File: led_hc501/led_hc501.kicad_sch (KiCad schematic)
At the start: 14 parts, among them J1 LED02, J10 Conn_01x03_Pin, J11 BATTERY, J2 Conn_01x01_Pin, J3 Conn_01x01_Pin, J4 BUZZ, J5 LED01, J6 HC-SR501_01, J7 Conn_01x01_Pin, J8 Conn_01x01_Pin, J9 LED03, Q3 IRLZ44N

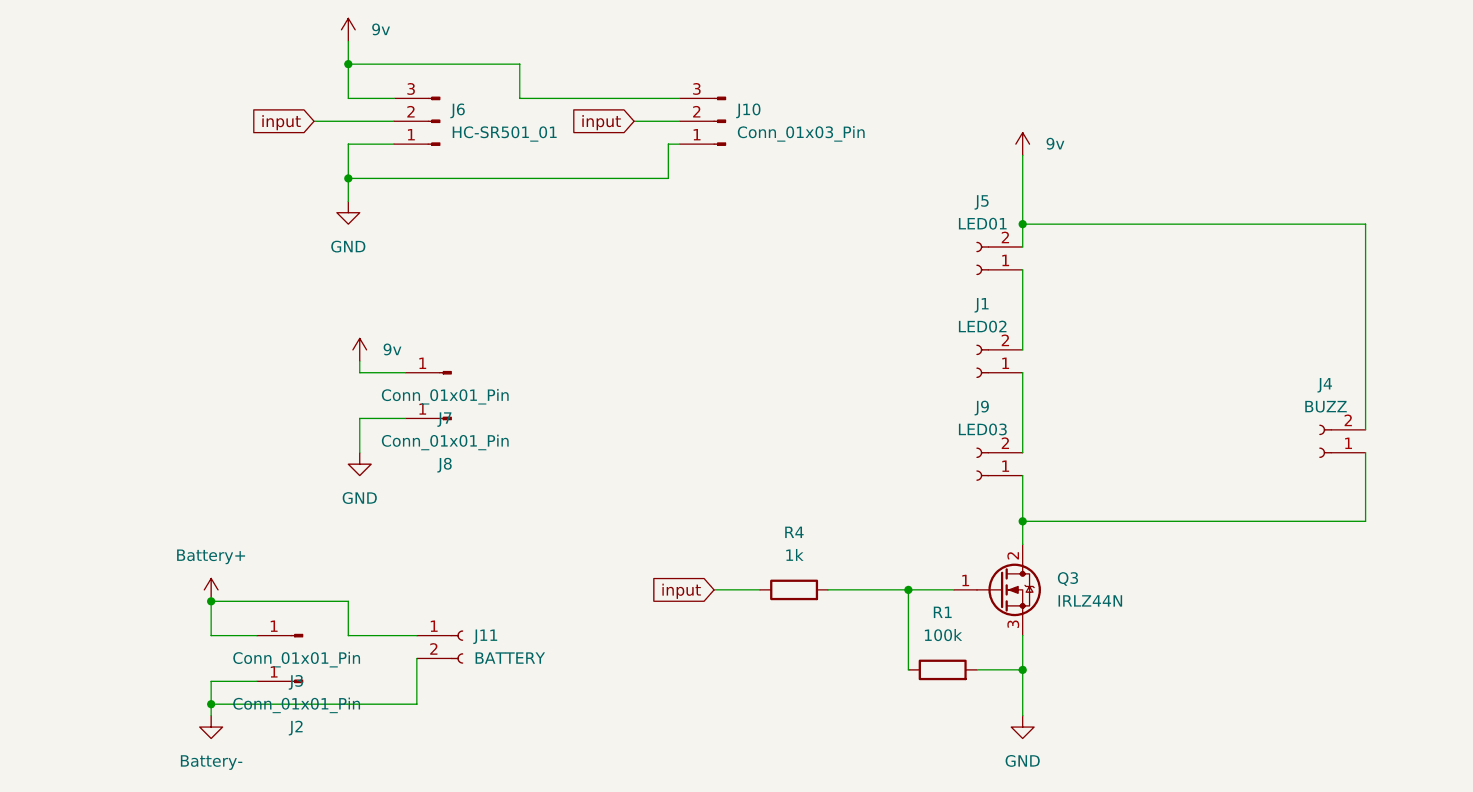
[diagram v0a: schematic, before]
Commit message: [SCHEMATIC] testing
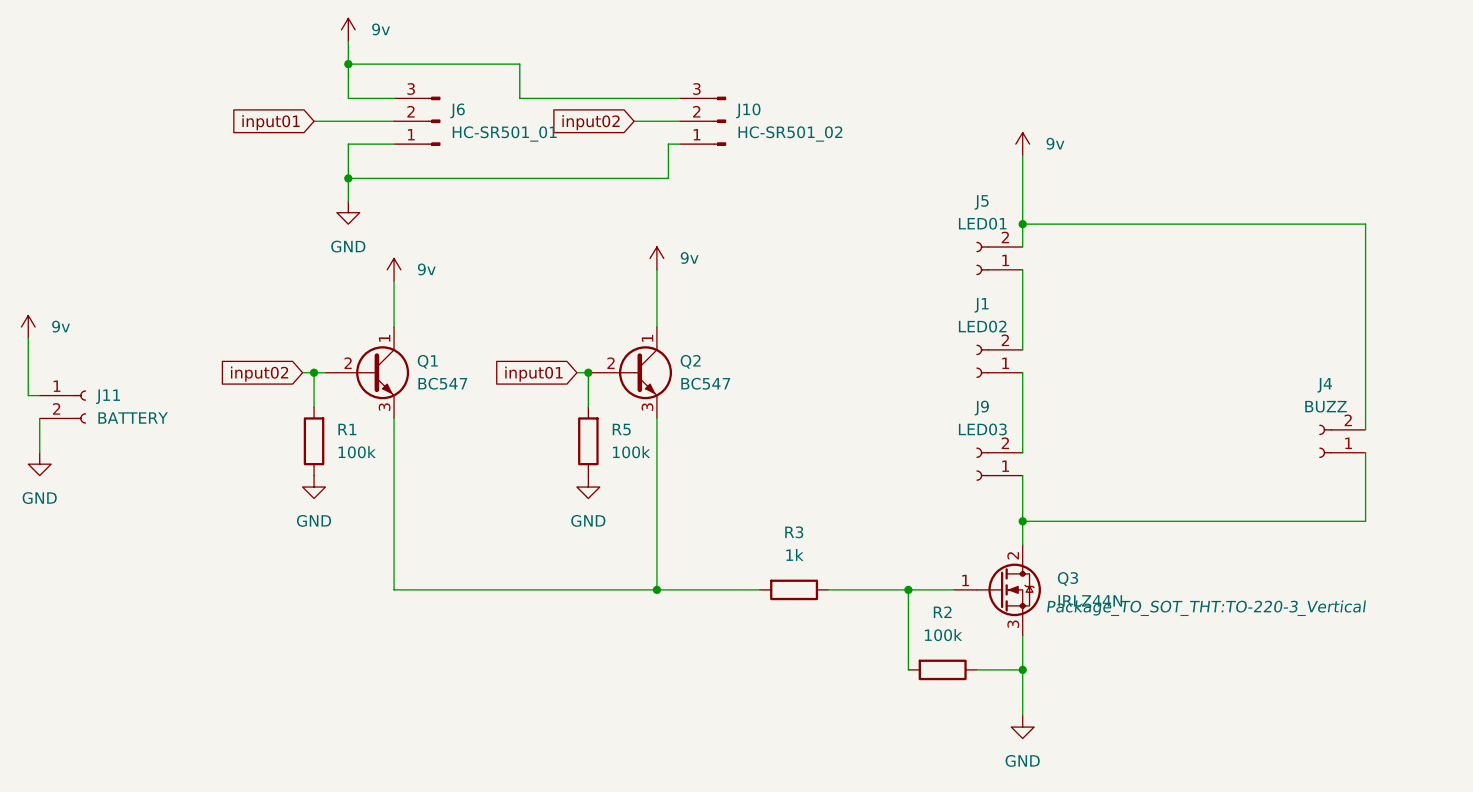
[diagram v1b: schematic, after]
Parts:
- removed J2, J3, J7, J8: Conn_01x01_Pin, Connector_PinHeader_2.54mm:PinHeader_1x01_P2.54mm_Vertical, symbol Connector:Conn_01x01_Pin
- removed R4: 1k, Resistor_THT:R_Axial_DIN0309_L9.0mm_D3.2mm_P2.54mm_Vertical, symbol Device:R
- added Q1, Q2: BC547, Package_TO_SOT_THT:TO-92L_Inline_Wide, symbol Transistor_BJT:BC547
- added R2, R5: 100k, Resistor_THT:R_Axial_DIN0207_L6.3mm_D2.5mm_P7.62mm_Horizontal, symbol Device:R
- added R3: 1k, Resistor_THT:R_Axial_DIN0207_L6.3mm_D2.5mm_P7.62mm_Horizontal, symbol Device:R
- J10: value Conn_01x03_Pin -> HC-SR501_02
- R1: footprint Resistor_THT:R_Axial_DIN0309_L9.0mm_D3.2mm_P2.54mm_Vertical -> Resistor_THT:R_Axial_DIN0207_L6.3mm_D2.5mm_P7.62mm_Horizontal
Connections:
- net Battery+ is gone; now on net 9v: J11.1 (Pin_1)
- net Battery- is gone; now on net GND: J11.2 (Pin_2)
- net 9v: now also Q1.1 (C), Q2.1 (C)
- net GND: now also R1.1, R2.1, R5.1; no longer R1.2
- net at Q3.1 (G): now also R2.2, R3.1; no longer R1.1
- net input renamed input01
- net input01: now also Q2.2 (B), R5.2; no longer J10.2 (Pin_2)
- new net: Q1.3 (E), Q2.3 (E), R3.2
- new net input02: J10.2 (Pin_2), Q1.2 (B), R1.2
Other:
- moved on the sheet: J11
